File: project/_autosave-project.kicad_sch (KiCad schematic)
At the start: 20 parts, among them J1 Conn_02x16_Odd_Even, J2 TYPE-C 6P(040新), Q1 PMOS, Q2 NPN, Q3 NPN, Q4 PMOS, SW1 SS-12D10L9, U2 CH224K

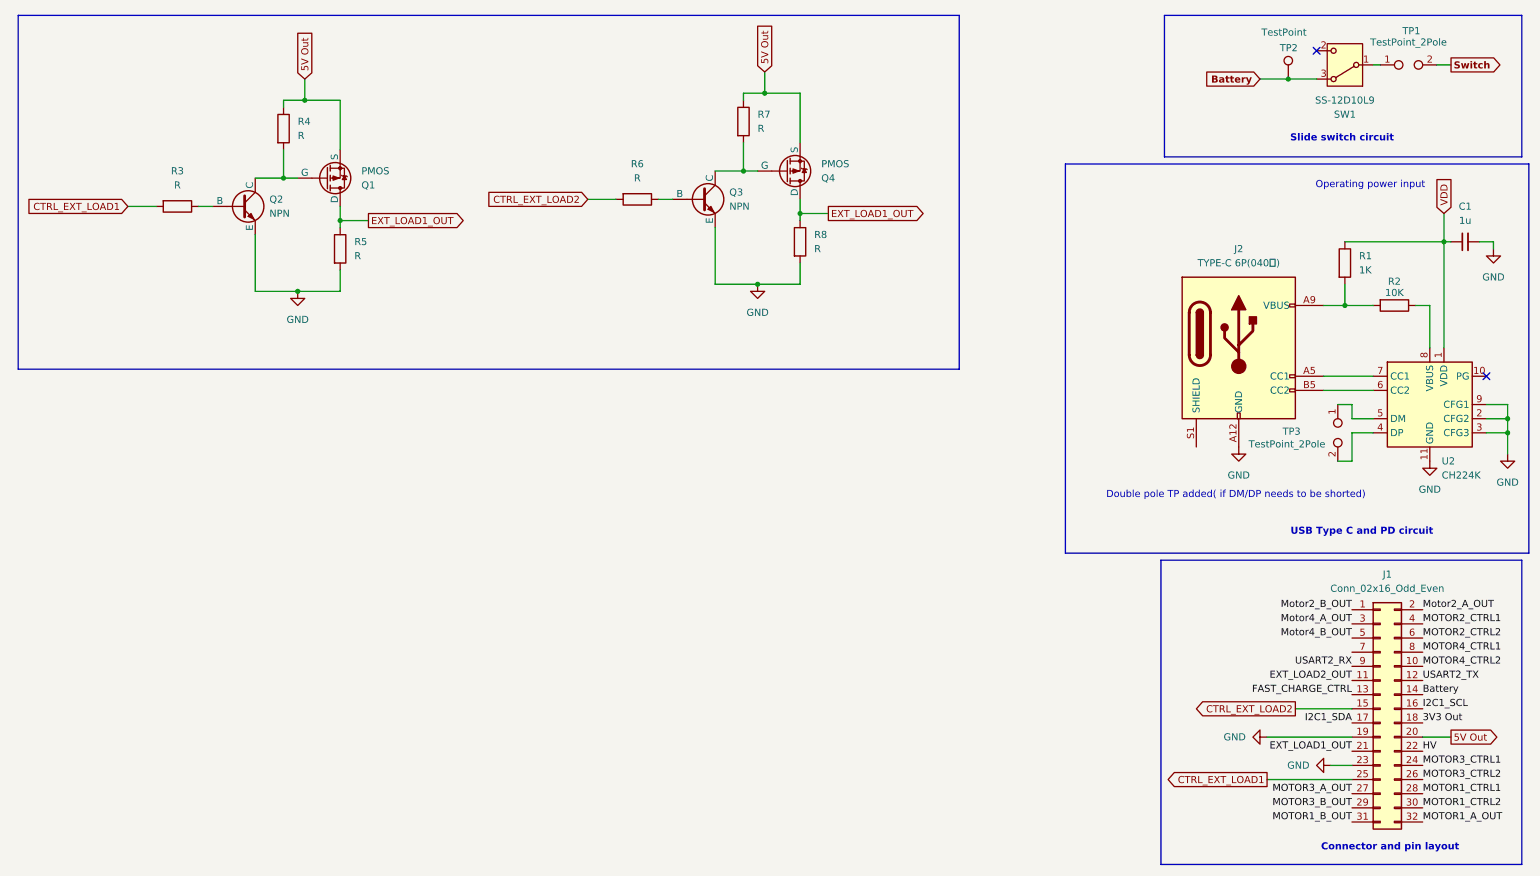
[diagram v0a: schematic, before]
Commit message: Update _autosave-project.kicad_sch
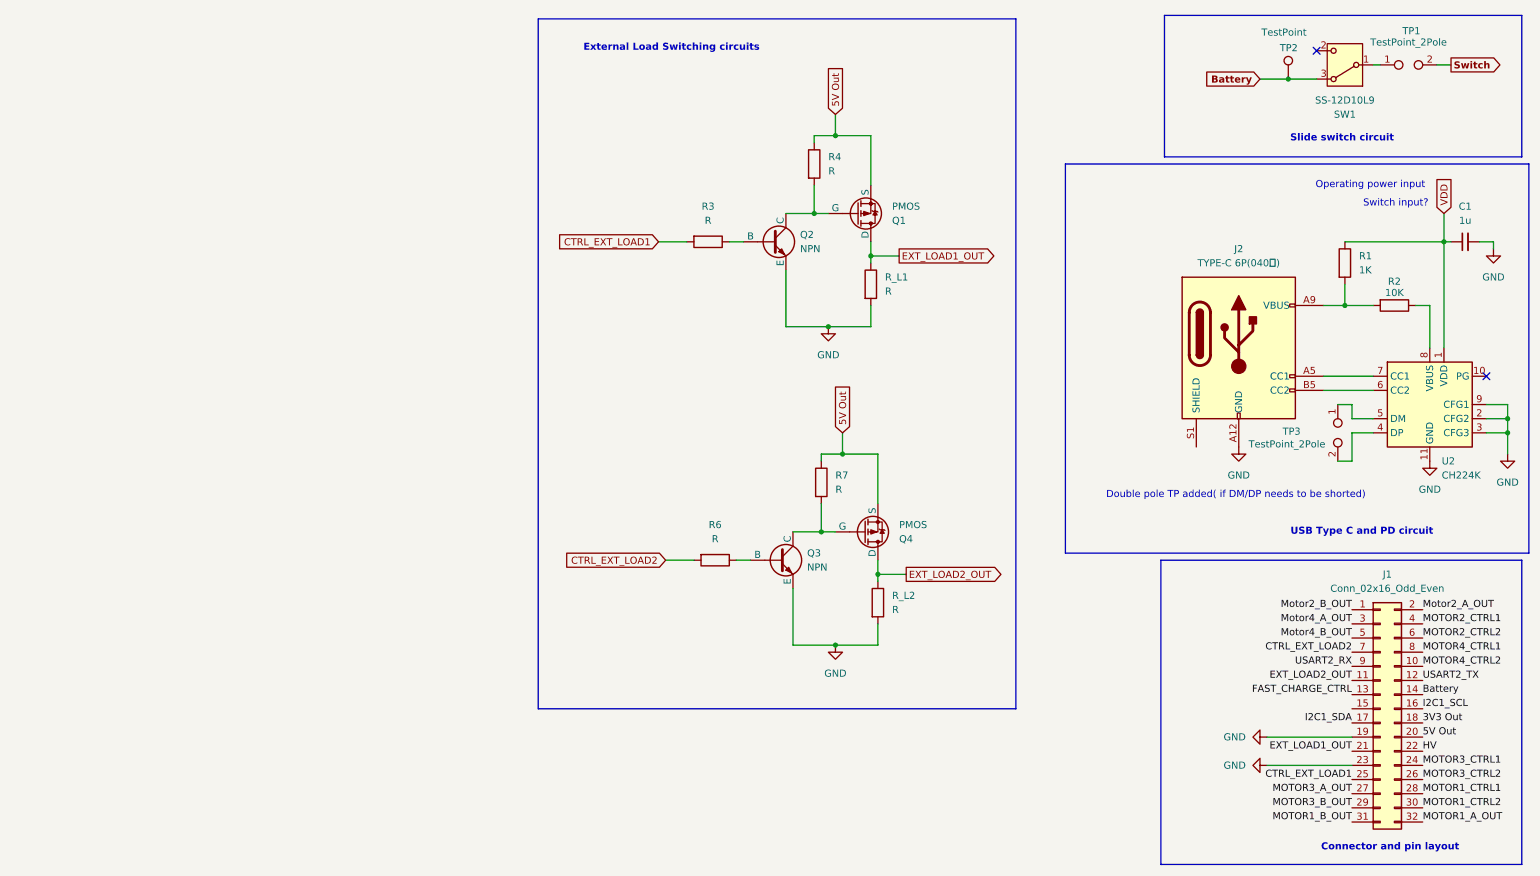
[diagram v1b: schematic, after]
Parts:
- renumbered R5 to R_L1, R8 to R_L2
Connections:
- net CTRL_EXT_LOAD2: now also J1.7 (Pin_7); no longer J1.15 (Pin_15)
- net EXT_LOAD1_OUT: no longer Q4.1 (D), R_L2.1
- net EXT_LOAD2_OUT: now also Q4.1 (D), R_L2.1
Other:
- note added: "External Load Switching circuits"
- note added: "Switch input?"
- moved on the sheet: Q1, Q2, Q3, Q4, R3, R4, R6, R7, R_L1, R_L2
